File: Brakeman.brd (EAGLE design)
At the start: 37.3 x 48.3 mm, 9 parts

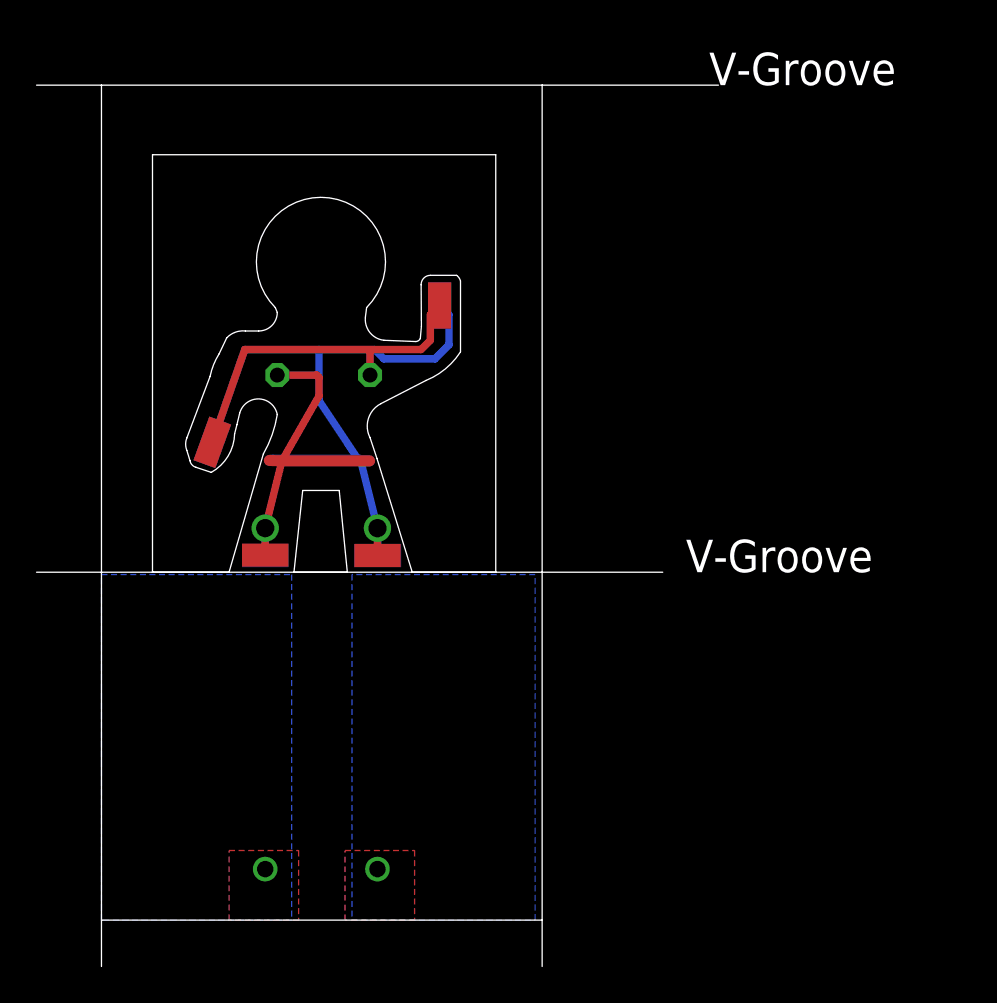
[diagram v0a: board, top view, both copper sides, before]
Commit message: Version 2.4
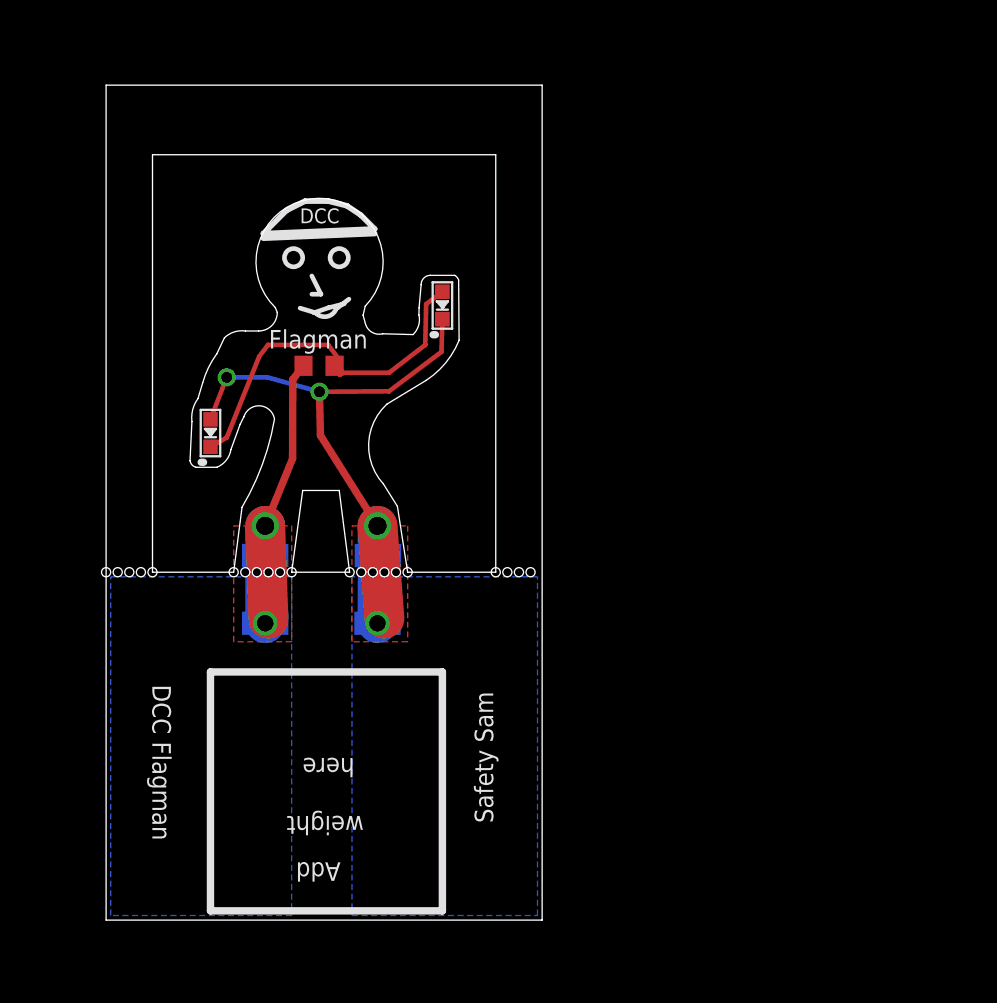
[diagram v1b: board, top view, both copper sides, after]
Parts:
- removed PADL1, PADL2, PADNA, PADNA2, PADNF2, PADSF2: pad, wirepad:SMD1.27-2.54
- removed R1: 1k0, resistor:0204/5
- added LED1, LED2: (no value), SPCoast:0603-LED
- added PADNF1, PADSF1: pad, SPCoast:SMD1,27-2,54
- added R1K: 1k0, resistor:R0603
- PADNF, PADSF: device wirepad:SMD1.27-2.54 -> SPCoast:SMD1,27-2,54
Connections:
- net LIMITED: now also LED1.C, LED2.A, R1K.1; no longer PADL1.1, PADL2.1, R1.1
- net N: now also LED1.A, LED2.C, PADNF1.1; no longer PADNA.1, PADNA2.1, PADNF2.1
- net S: now also PADSF1.1, R1K.2; no longer PADSF2.1, R1.2
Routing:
- net N: track 38.6 -> 35.5 mm, vias 2 -> 4
- net LIMITED: track 19.3 -> 21.3 mm
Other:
- board size 37.3 x 48.3 mm -> 23.9 x 45.7 mm
- board text added: "2016.11 2024.01"
- board text added: "John Plocher 2024.01"
- board text added: "Safety Sam DCC Flagman"
- board text removed: "2016.11"
- board text removed: "V-Groove"
